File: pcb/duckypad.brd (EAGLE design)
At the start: 110 x 96 mm, 98 parts, among them IC2 REG1117, SW1 SPST_TACT-EVQQ2, SW2 SPST_TACT-EVQQ2, SW21 EC12E_SW, SW22 EC12E_SW, SW3 324_SW324_SWITCH_FOOT_HOLE, U1 USBC_16P, U2 USBC_16P, U3 ESP32-S3FN8, Y1 16MHz_12pF

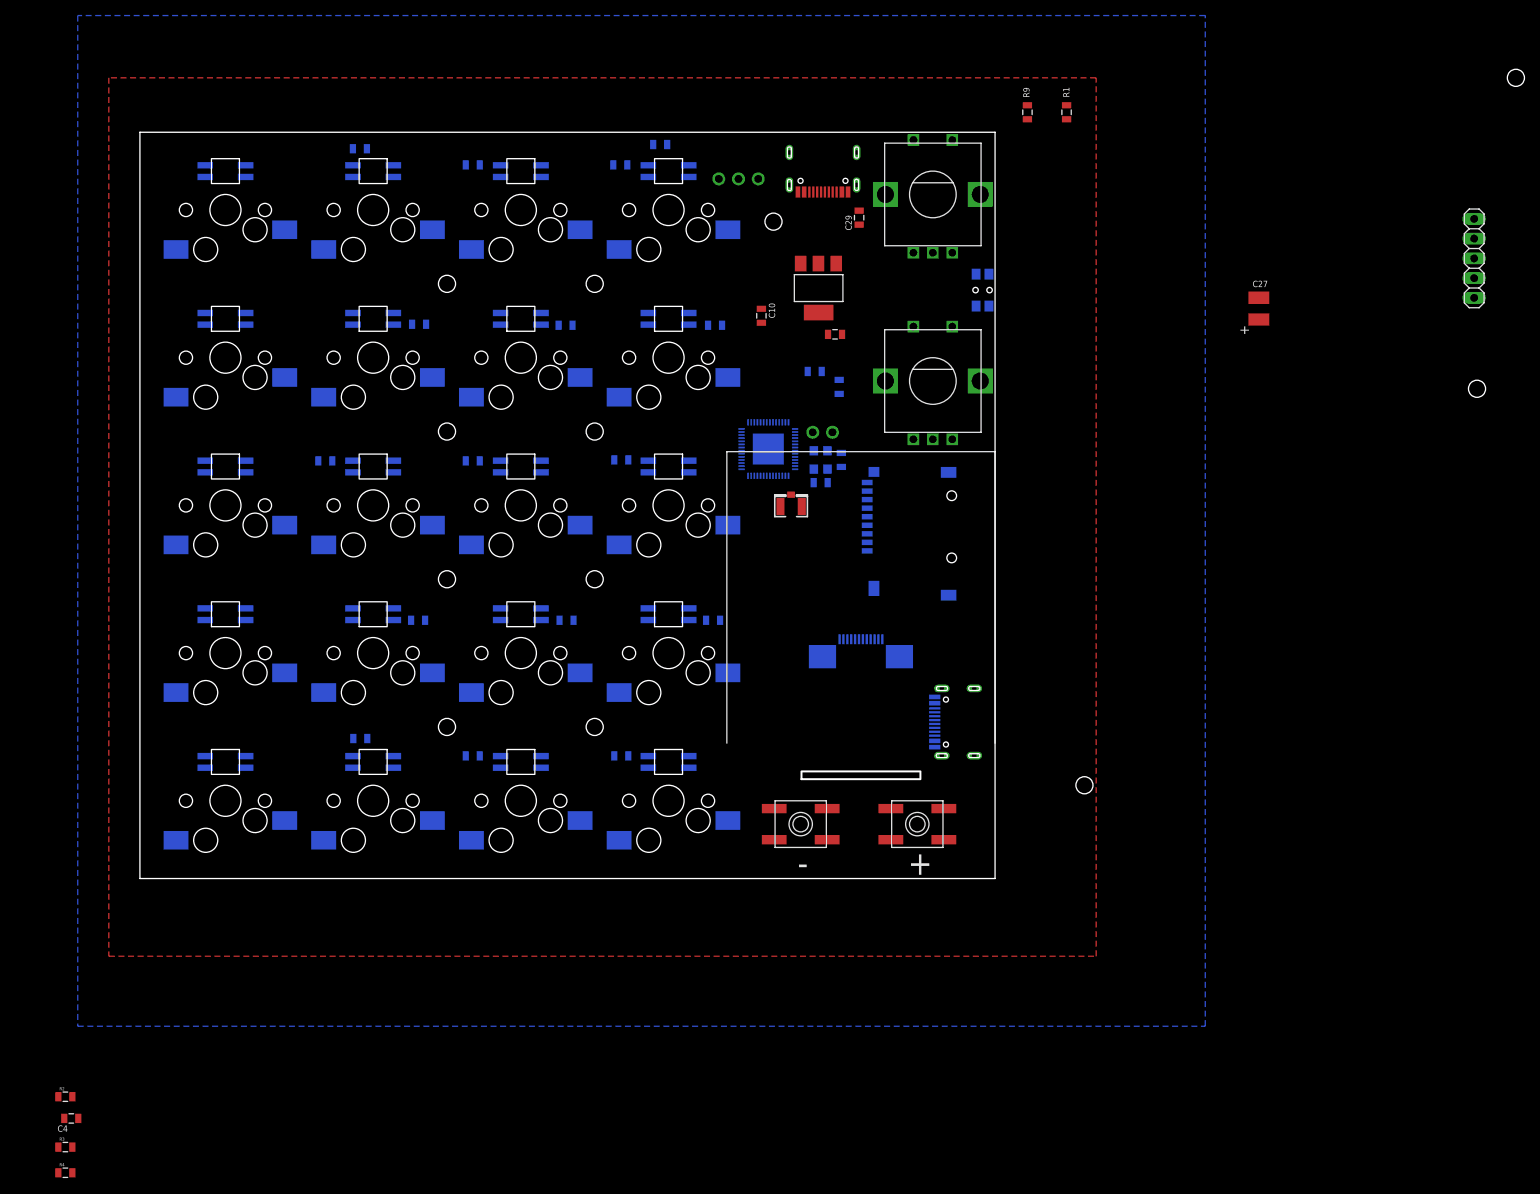
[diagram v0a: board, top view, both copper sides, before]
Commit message: working on pcb
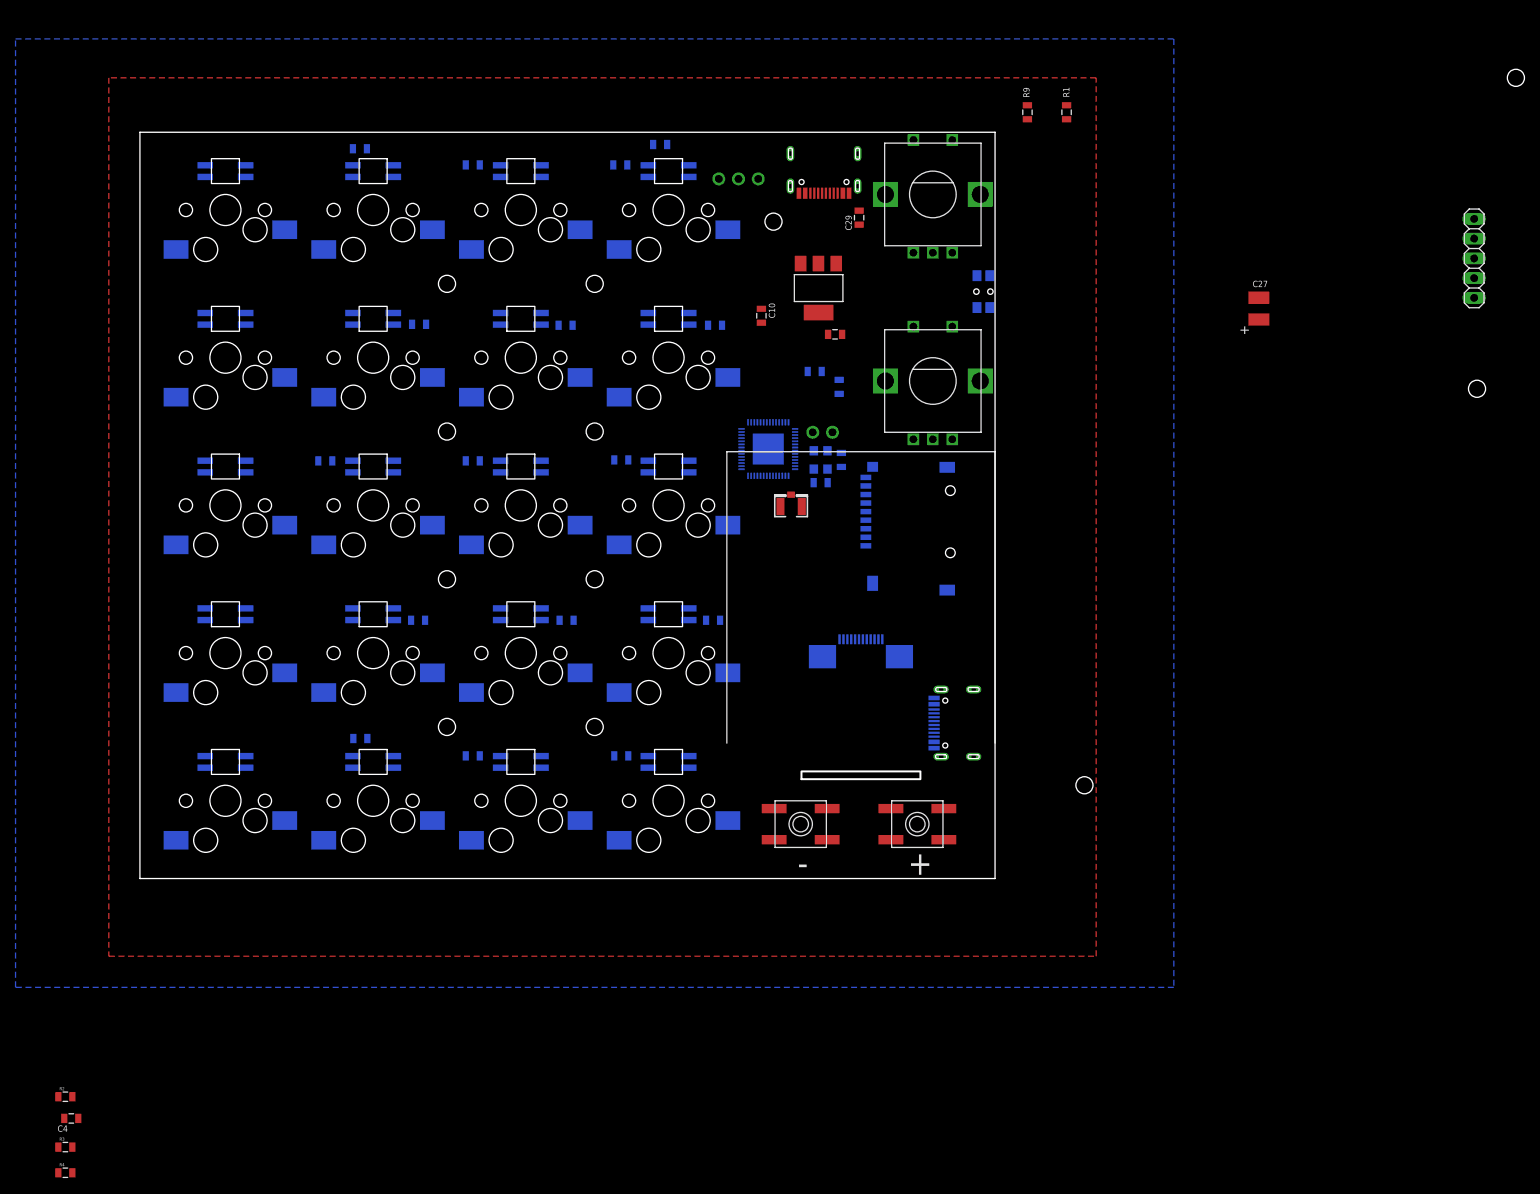
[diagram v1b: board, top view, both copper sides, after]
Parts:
- moved SD1 0.68 mm to (81.0, 45.0)
- moved SW3 0.22 mm to (88.5, 75.5)
- moved U2 0.20 mm to (68.0, 92.0)
- moved U1 0.16 mm to (86.0, 20.0)
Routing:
- added copper zone on layer 16, net GND
- removed copper zone on layer 16, net +3V3
